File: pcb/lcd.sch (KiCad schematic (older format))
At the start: 32 parts, among them J500 FPC_18P_1.0MM, U100 MCIMX7S5EVM08SC, U500 XC2C32A_QF32, U501 LT1617, U502 LM324

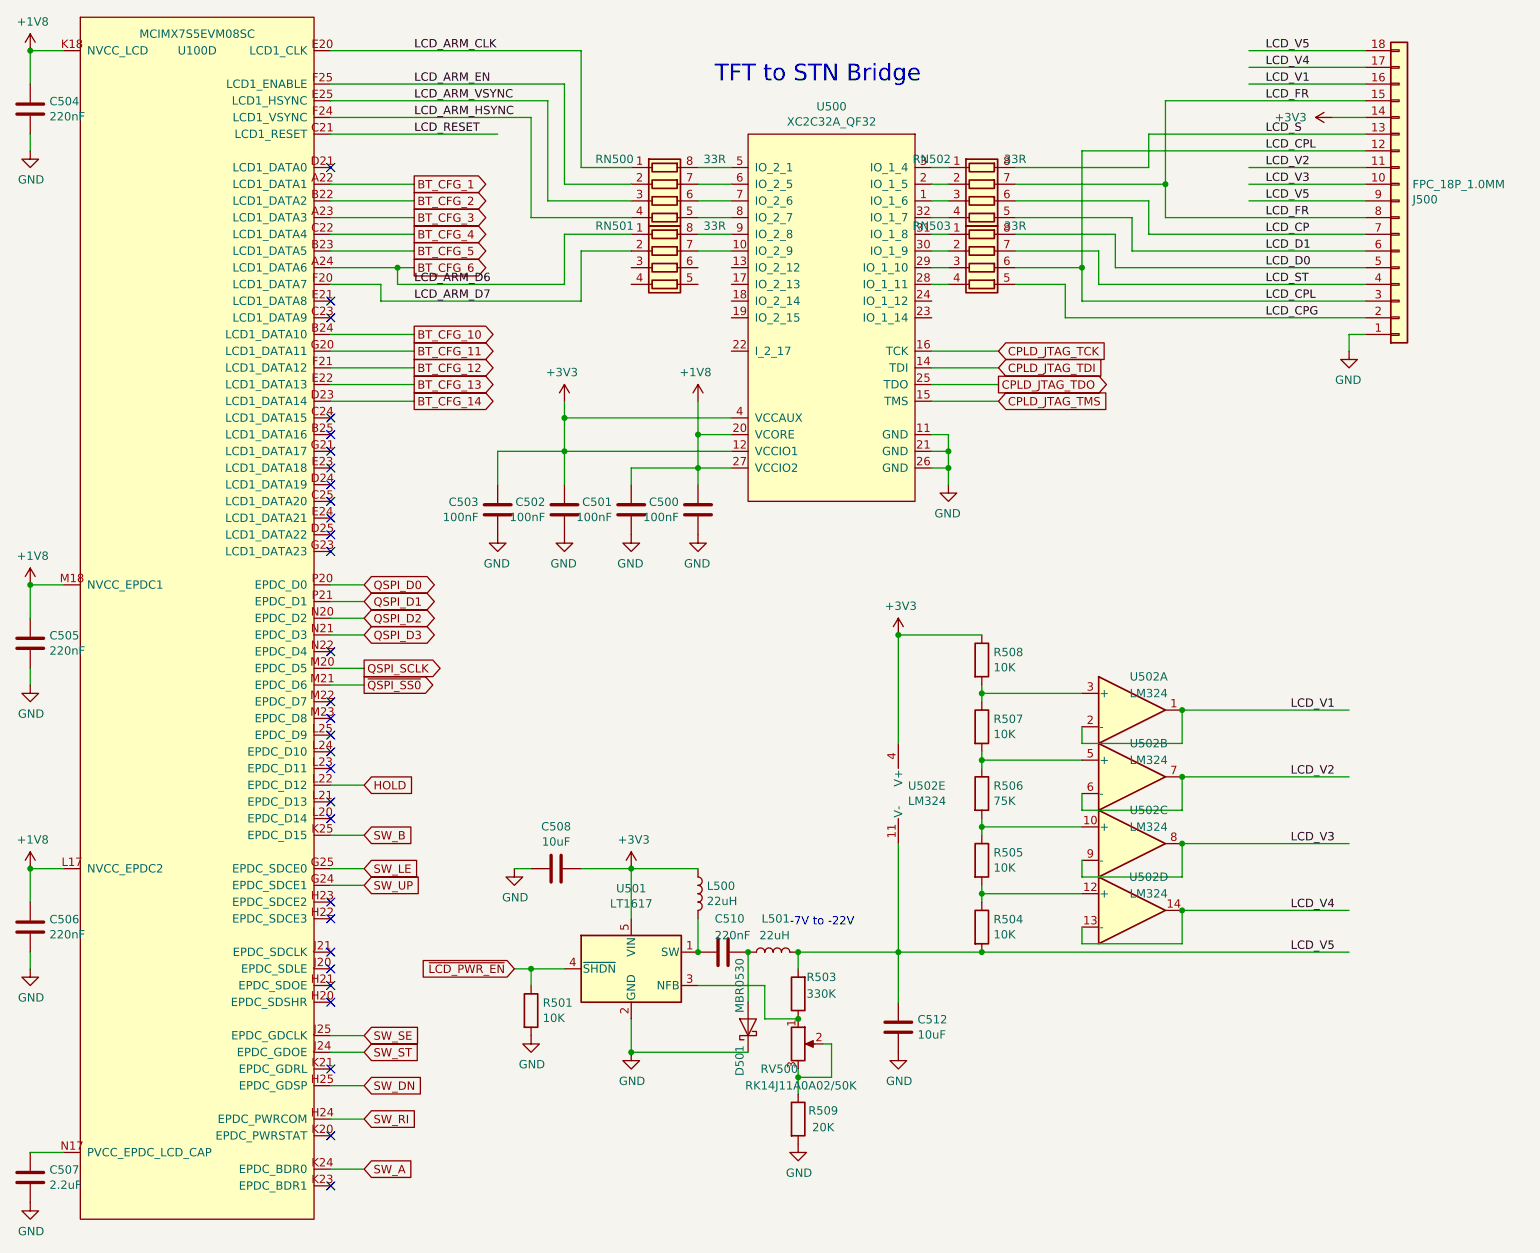
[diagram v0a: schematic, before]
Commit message: pcb: rev 0.1
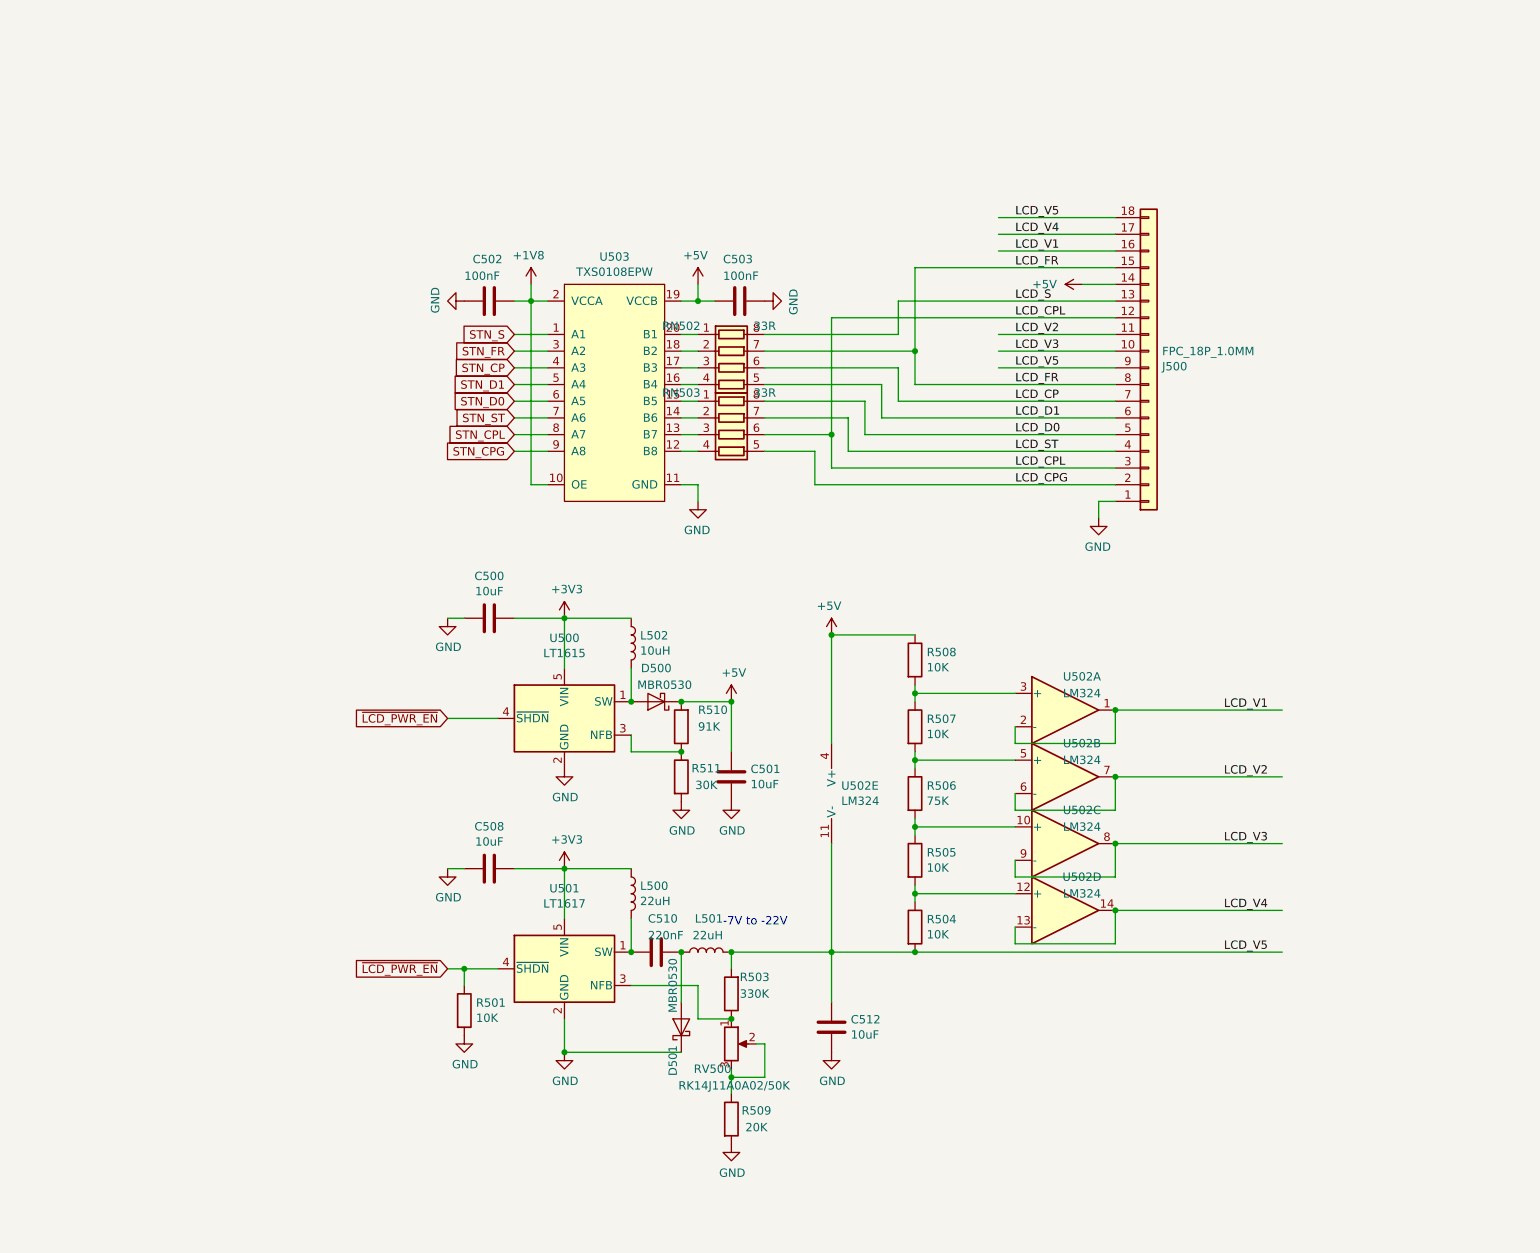
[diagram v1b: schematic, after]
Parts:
- removed C504, C505, C506: 220nF, Capacitor_SMD:C_0402_1005Metric, symbol Device:C
- removed C507: 2.2uF, Capacitor_SMD:C_0402_1005Metric, symbol Device:C
- removed RN500, RN501: 33R, Resistor_SMD:R_Array_Convex_4x0402, symbol Device:R_Pack04
- removed U100: MCIMX7S5EVM08SC, footprints:BGA-541_25x25_19.0x19.0mm, symbol symbols:MCIMX7S5EVM08SC
- removed U500: XC2C32A_QF32, Package_DFN_QFN:QFN-32-1EP_5x5mm_P0.5mm_EP3.1x3.1mm, symbol symbols:XC2C32A_QF32
- added D500: MBR0530, Diode_SMD:D_SOD-123, symbol Device:D_Schottky
- added L502: 10uH, Inductor_SMD:L_Vishay_IHLP-1212, symbol Device:L
- added R510: 91K, Resistor_SMD:R_0603_1608Metric, symbol Device:R
- added R511: 30K, Resistor_SMD:R_0603_1608Metric, symbol Device:R
- added U500: LT1615, Package_TO_SOT_SMD:TSOT-23-5, symbol symbols:LT1615
- added U503: TXS0108EPW, Package_SO:TSSOP-20_4.4x6.5mm_P0.65mm, symbol symbols:TXS0108EPW
- C500, C501: value 100nF -> 10uF; footprint Capacitor_SMD:C_0402_1005Metric -> Capacitor_SMD:C_0603_1608Metric
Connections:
- net labels added: +5V, STN_CP, STN_CPG, STN_CPL, STN_D0, STN_D1, STN_FR, STN_S, STN_ST
- net labels removed: BT_CFG_1, BT_CFG_10, BT_CFG_11, BT_CFG_12, BT_CFG_13, BT_CFG_14, BT_CFG_2, BT_CFG_3, BT_CFG_4, BT_CFG_5, BT_CFG_6, CPLD_JTAG_TCK, CPLD_JTAG_TDI, CPLD_JTAG_TDO, CPLD_JTAG_TMS, HOLD, LCD_ARM_CLK, LCD_ARM_D6, LCD_ARM_D7, LCD_ARM_EN, LCD_ARM_HSYNC, LCD_ARM_VSYNC, LCD_RESET, QSPI_D0, QSPI_D1, QSPI_D2, QSPI_D3, QSPI_SCLK, SW_A, SW_B, SW_DN, SW_LE, SW_RI, SW_SE, SW_ST, SW_UP, ~QSPI_SS0
- wire segments 189 -> 128
- no-connect marks 29 -> 0
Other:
- note removed: "TFT to STN Bridge"
- moved on the sheet: C508, C510, C512, D501, J500, L500, L501, R501, R503, R504, R505, R506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
